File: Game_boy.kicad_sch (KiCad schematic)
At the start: 63 parts, among them J1 USB_C_Receptacle_USB2.0_14P, J2 Conn_01x11, J3 Conn_01x04, SW1 SW_Push, SW2 SW_Push, SW3 SW_Push, SW4 SW_Push, SW5 SW_Push, SW6 SW_Push, SW7 SW_Push, SW8 SW_Push, SW9 SW_Push, U1 RT6154AGQW, U2 W25Q64JVXGIQ, U3 RP2040, Y1 12 MHz

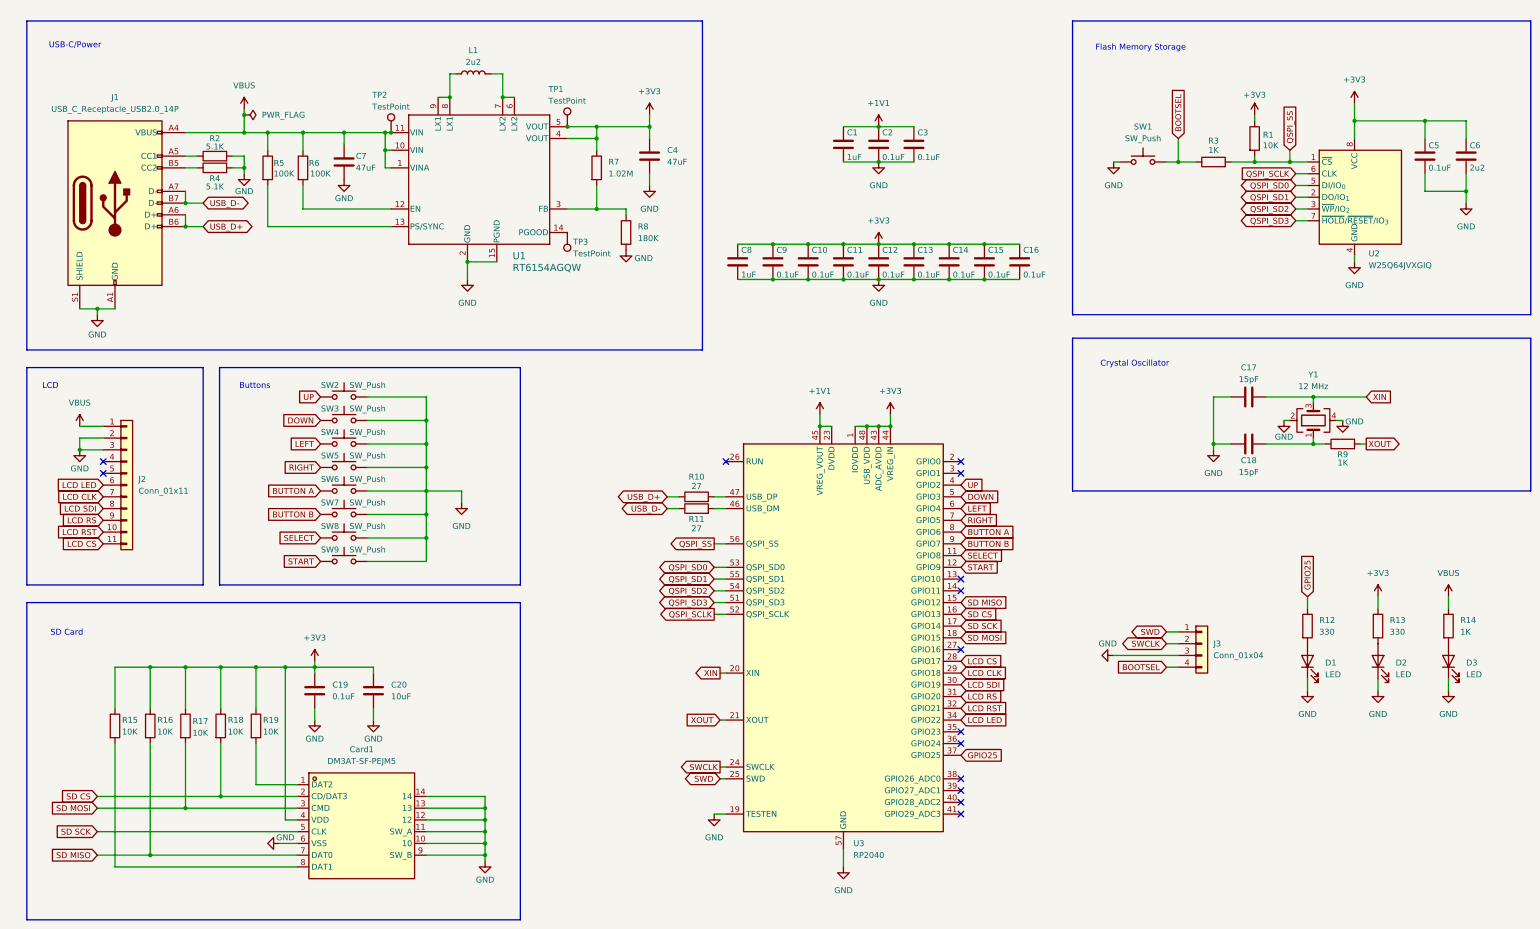
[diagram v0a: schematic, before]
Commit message: Update Readme
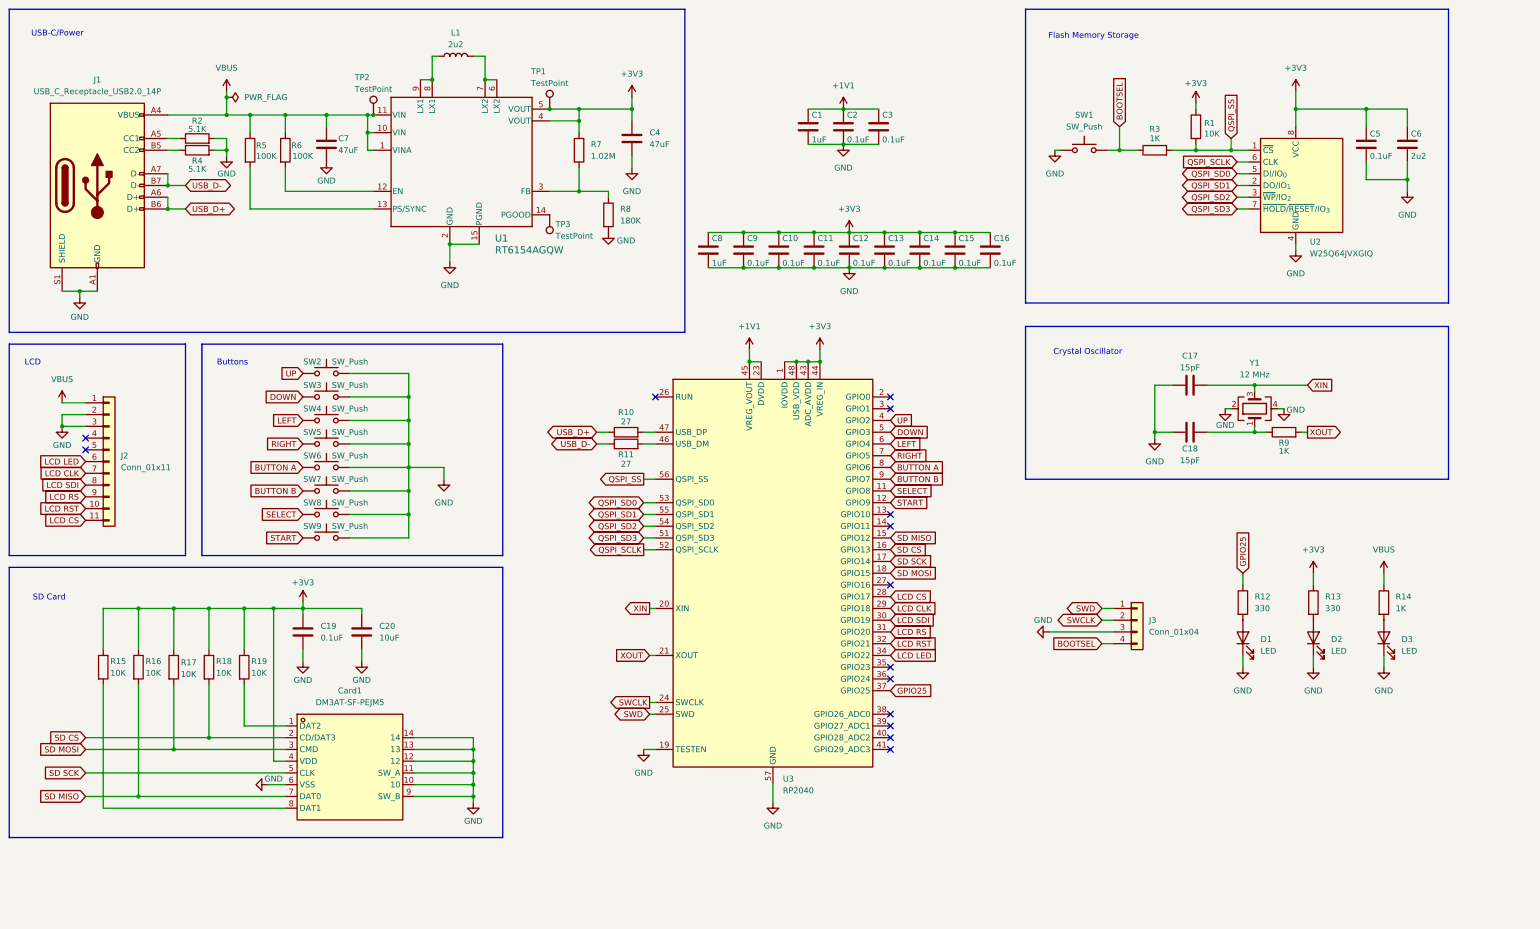
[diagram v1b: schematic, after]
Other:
- title: (none) -> Gameboy
- moved on the sheet: C1, C10, C11, C12, C13, C14, C15, C16, C17, C18, C19, C2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
